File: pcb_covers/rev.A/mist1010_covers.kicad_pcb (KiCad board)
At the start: 2 copper layers, 133.5 x 61.5 mm, 1 part

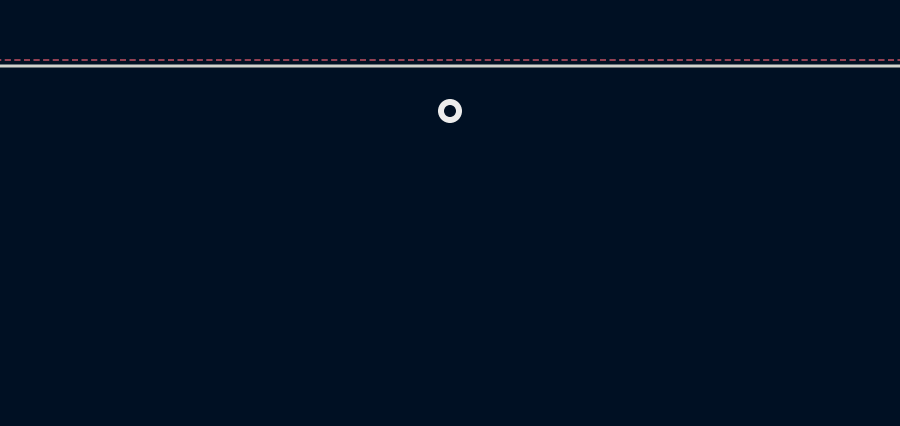
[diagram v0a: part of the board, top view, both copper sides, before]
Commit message: update pcb rev.A
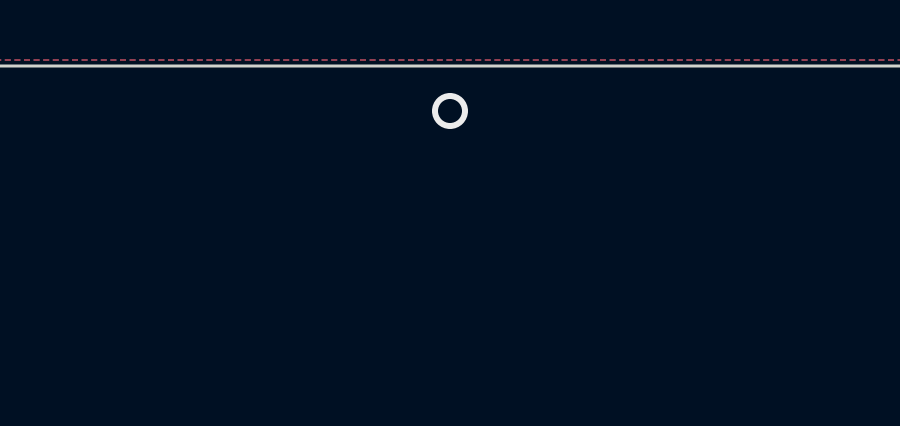
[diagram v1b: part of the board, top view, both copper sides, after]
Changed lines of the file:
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@@
     (style (thickness 0.15) (arrow_length 1.27) (text_position_mode 0) (extension_height 0.58642) (extension_offset 0.5) keep_text_aligned)
   )
-  (via (at 144.5 63) (size 0.8) (drill 0.4) (layers "F.Cu" "B.Cu") (free) (net 1))
+  (via (at 144.5 63) (size 1.2) (drill 0.8) (layers "F.Cu" "B.Cu") (free) (net 1))
   (zone (net 1) (net_name "COMMON") (layers F&B.Cu) (hatch edge 0.508)
     (connect_pads (clearance 0.508))
